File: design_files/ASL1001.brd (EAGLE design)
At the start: 8 x 4 mm, 5 parts

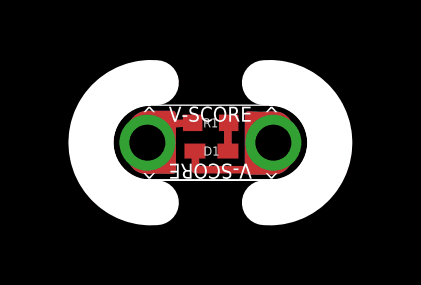
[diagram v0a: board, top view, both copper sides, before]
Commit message: update format
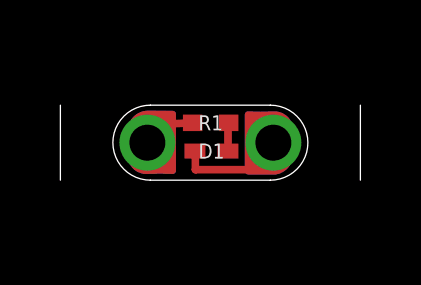
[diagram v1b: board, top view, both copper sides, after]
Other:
- board size 8 x 4 mm -> 10 x 2.5 mm
- board text added: "3"
- board text removed: "2"
- board text removed: "^ V-SCORE ^"
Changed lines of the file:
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@@
 <setting verticaltext="up"/>
 </settings>
-<grid distance="1.5" unitdist="mm" unit="mm" style="lines" multiple="1" display="yes" altdistance="0.025" altunitdist="inch" altunit="inch"/>
+<grid distance="0.1" unitdist="mm" unit="mm" style="lines" multiple="1" display="yes" altdistance="0.05" altunitdist="mm" altunit="mm"/>
 <layers>
 <layer number="1" name="Top" color="4" fill="1" visible="yes" active="yes"/>
@@
 <wire x1="69.85" y1="50.8" x2="0" y2="50.8" width="0.127" layer="48"/>
 <wire x1="0" y1="50.8" x2="0" y2="0" width="0.127" layer="48"/>
-<dimension x1="23.25" y1="20" x2="16.75" y2="20" x3="20" y3="26.224653125" layer="48"/>
+<dimension x1="23.25" y1="21.25" x2="16.75" y2="21.25" x3="20" y3="27.474653125" layer="48"/>
 <text x="48.111025" y="4.365003125" size="0.889" layer="48">TinyLily LED - 0402</text>
 <text x="44.986825" y="1.7714" size="0.889" layer="48">AS-PCB-ASL1001</text>
-<text x="67.3810375" y="1.6952" size="0.889" layer="48">2</text>
+<text x="67.3810375" y="1.6952" size="0.889" layer="48">3</text>
 <text x="19.54081875" y="19.118715625" size="0.762" layer="22" rot="MR0">-</text>
 <text x="21.0168625" y="20.145540625" size="0.762" layer="22" rot="MR0">+</text>
-<dimension x1="18" y1="21.25" x2="18" y2="18.75" x3="10.150421875" y3="20" layer="48"/>
-<wire x1="21.8" y1="22" x2="21.8" y2="18" width="1.5" layer="46" curve="-190"/>
+<dimension x1="16.75" y1="21.25" x2="16.75" y2="18.75" x3="8.900421875" y3="20" layer="48"/>
 <text x="40.5384" y="14.481796875" size="0.4572" layer="48" ratio="10">Released under the Creative Commons Attribution Share-Alike 3.0 License</text>
 <text x="40.5384" y="13.719796875" size="0.4572" layer="48" ratio="10">http://creativecommons.org/licenses/by-sa/3.0</text>
 <text x="40.5384" y="12.449796875" size="0.4572" layer="48" ratio="10">Original Arduino Uno Design by Team Arduino</text>
 <text x="40.5384" y="11.687796875" size="0.4572" layer="48" ratio="10">LilyPad Arduino Design by Leah Buechley and Sparkfun Electronics</text>
-<wire x1="18.2" y1="18" x2="18.2" y2="22" width="1.5" layer="46" curve="-190"/>
 <wire x1="18" y1="21.25" x2="18" y2="18.75" width="0.0254" layer="20" curve="180"/>
 <wire x1="22" y1="18.75" x2="22" y2="21.25" width="0.0254" layer="20" curve="180"/>
 <wire x1="22" y1="21.25" x2="18" y2="21.25" width="0.0254" layer="20"/>
-<wire x1="16.75" y1="21.25" x2="18" y2="21.25" width="0.0254" layer="20"/>
 <wire x1="18" y1="18.75" x2="22" y2="18.75" width="0.0254" layer="20"/>
-<wire x1="18" y1="21.25" x2="18" y2="18.75" width="0.0254" layer="108" curve="180"/>
-<wire x1="22" y1="18.75" x2="22" y2="21.25" width="0.0254" layer="108" curve="180"/>
-<wire x1="22" y1="21.25" x2="18" y2="21.25" width="0.0254" layer="108"/>
-<wire x1="18" y1="18.75" x2="22" y2="18.75" width="0.0254" layer="108"/>
 <text x="40.5384" y="10.976596875" size="0.4572" layer="48" ratio="10">TinyDuino, TinyLily and TinyShield Designs by TinyCircuits</text>
-<text x="20" y="20.7" size="0.5" layer="20" align="bottom-center">^  V-SCORE  ^</text>
-<wire x1="16.75" y1="18.75" x2="23.25" y2="18.75" width="0.0254" layer="20"/>
-<wire x1="22" y1="21.25" x2="23.25" y2="21.25" width="0.0254" layer="20"/>
-<text x="20" y="19.3" size="0.5" layer="20" rot="SR180" align="bottom-center">^  V-SCORE  ^</text>
+<wire x1="15" y1="21.25" x2="15" y2="18.75" width="0.0254" layer="20"/>
+<wire x1="25" y1="21.25" x2="25" y2="18.75" width="0.0254" layer="20"/>
 </plain>
 <attributes>
